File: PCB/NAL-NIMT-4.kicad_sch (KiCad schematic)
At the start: 16 parts

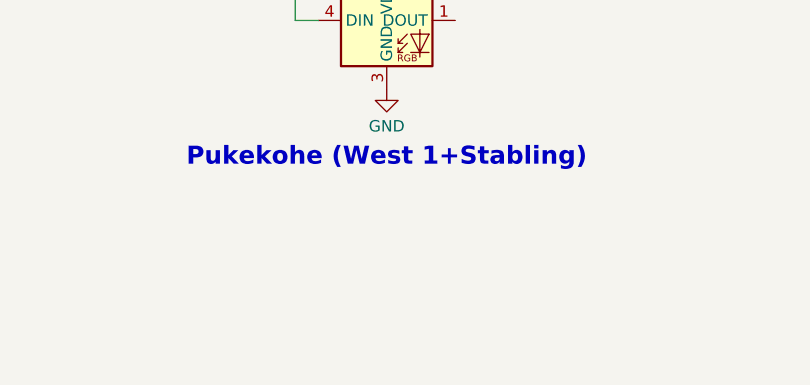
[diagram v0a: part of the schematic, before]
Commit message: PCB Checkpoint
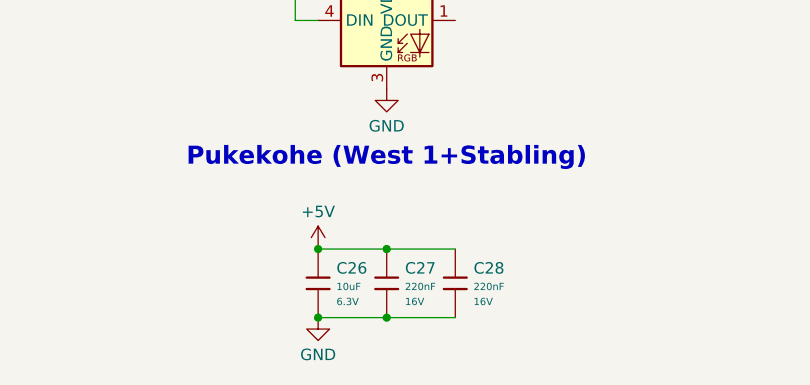
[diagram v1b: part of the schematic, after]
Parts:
- added C26: 10uF, PCM_JLCPCB:C_0402, symbol PCM_JLCPCB-Capacitors:0402,10uF
- added C27, C28: 220nF, PCM_JLCPCB:C_0402, symbol PCM_JLCPCB-Capacitors:0402,220nF
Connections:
- net +5V: now also C26.1, C27.1, C28.1
- net GND: now also C26.2, C27.2, C28.2
